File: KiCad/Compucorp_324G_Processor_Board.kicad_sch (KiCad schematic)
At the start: 9 parts, among them J5 Processor Interboard, J6 Test Connector, U5 TMC1872 (TCL07), U6 TMC1866 (TCL06), U7 TMC1867 (TCL05), U8 TMC1870 (TCL04)

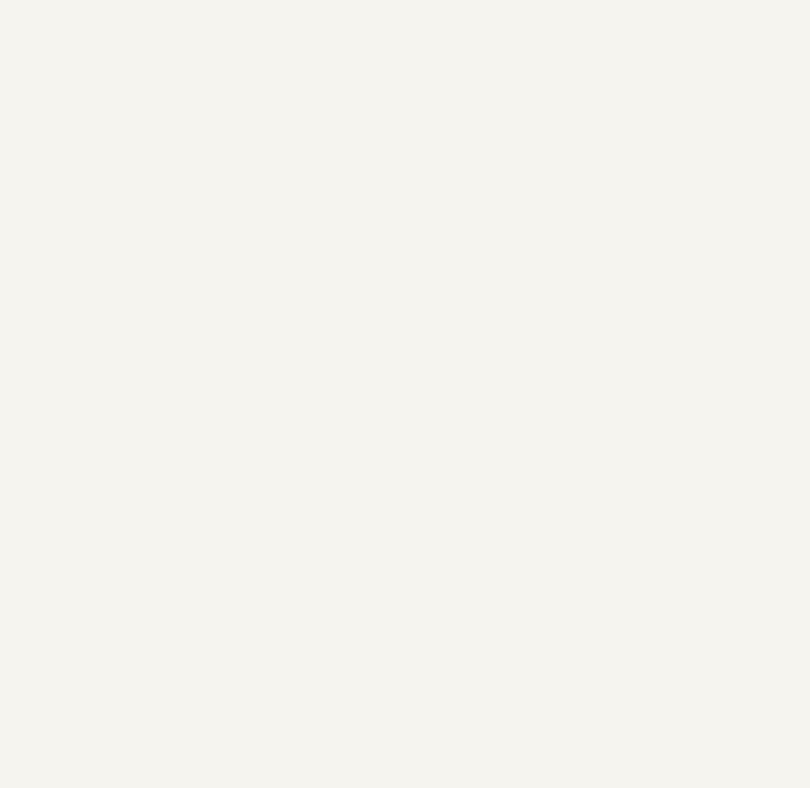
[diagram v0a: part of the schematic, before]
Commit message: Update Compucorp_324G_Processor_Board.kicad_sch
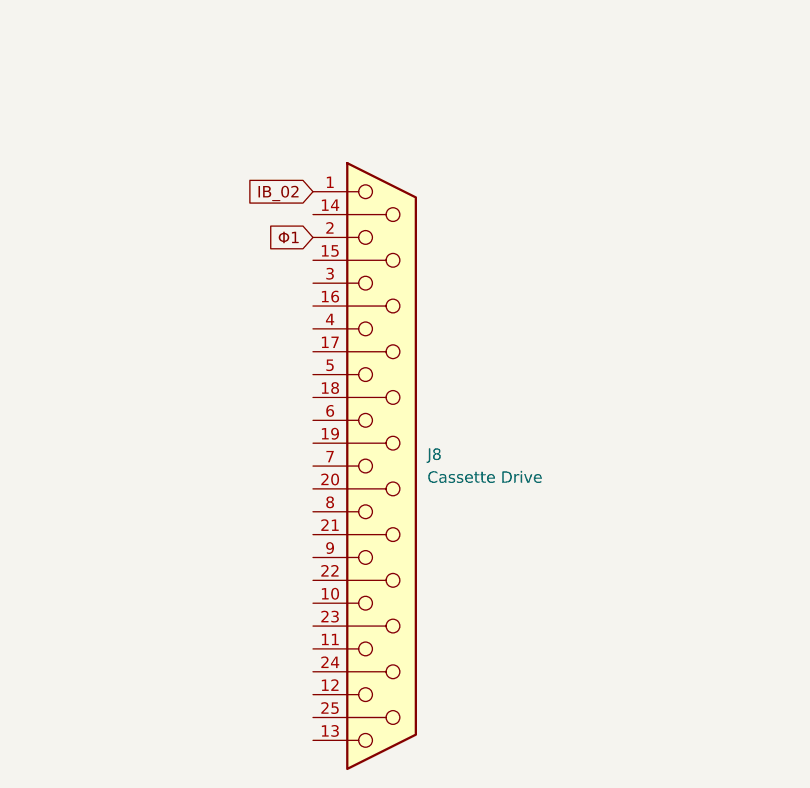
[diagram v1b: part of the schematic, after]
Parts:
- added J8: Cassette Drive, symbol Connector:DB25_Socket
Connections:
- net IB_02: now also J8.1
- net Φ1: now also J8.2
